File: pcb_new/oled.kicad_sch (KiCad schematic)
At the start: 33 parts, among them J10 3-2328724-1, U8 TPS6734ID

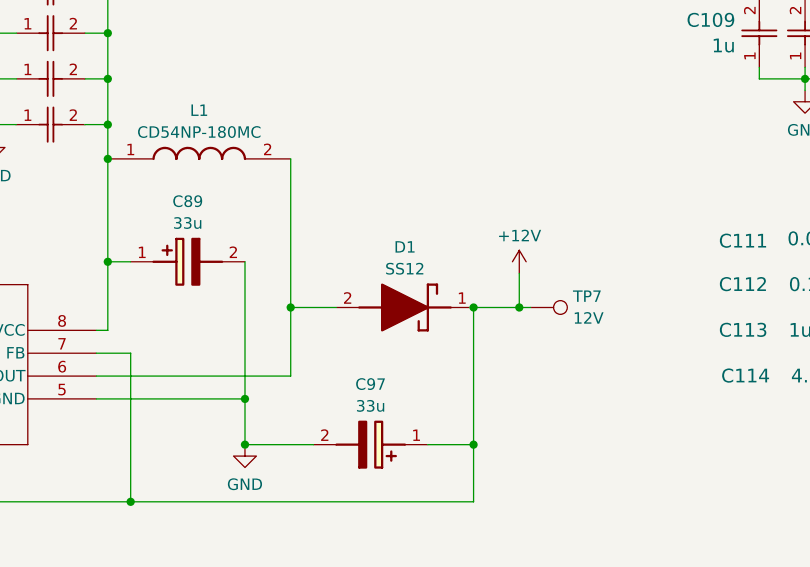
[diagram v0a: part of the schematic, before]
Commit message: initial test of new board
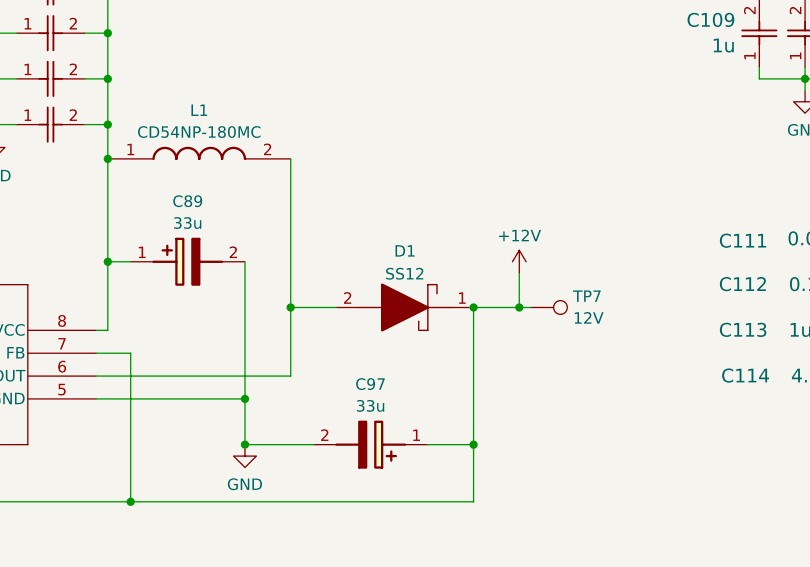
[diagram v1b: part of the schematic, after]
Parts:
- removed D1: SS12, OroLink:DIOM5027X244N, symbol OroLink:SS12
- added D1: SS12, OroLink:DIOM5027X244N, symbol SamacSys_Parts:SS12
- C105, C114, C115, C148: Mouser Part Number 81-GRM15C61E475ME15J -> (none)
- C89, C97: Mouser Part Number (none) -> 74-293D336X0020D2TE3; Mouser Price/Stock (none) -> https://www.mouser.de/ProductDetail/Vishay-Sprague/293D336X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
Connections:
- net +12V: now also D1.1
- net at L1.2, U8.6 (OUT): now also D1.2
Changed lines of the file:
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@@
 	)
 	(junction
-		(at 156.21 104.14)
-		(diameter 0)
-		(color 0 0 0 0)
-	)
-	(junction
 		(at 102.87 78.74)
 		(diameter 0)
@@
 	)
 	(junction
+		(at 156.21 104.14)
+		(diameter 0)
+		(color 0 0 0 0)
+	)
+	(junction
 		(at 243.84 120.65)
 		(diameter 0)
@@
 			)
 		)
-		(property "Mouser Part Number" "81-GRM15C61E475ME15J"
+		(property "Mouser Part Number" ""
 			(at 238.76 746.99 0)
 			(effects
@@
 	)
 	(symbol
-		(lib_id "OroLink:SS12")
-		(at 158.75 104.14 180)
-		(unit 1)
-		(exclude_from_sim no)
-		(in_bom yes)
-		(on_board yes)
-		(dnp no)
-		(fields_autoplaced yes)
-		(property "Reference" "D1"
-			(at 148.59 97.4555 0)
-			(effects
-				(font
-					(size 1.27 1.27)
-				)
-			)
-		)
-		(property "Value" "SS12"
-			(at 148.59 99.8798 0)
-			(effects
-				(font
-					(size 1.27 1.27)
-				)
-			)
-		)
-		(property "Footprint" "OroLink:DIOM5027X244N"
-			(at 146.05 10.49 0)
-			(effects
-				(font
-					(size 1.27 1.27)
-				)
-				(justify left top)
-				(hide yes)
-			)
-		)
-		(property "Datasheet" "https://www.panjit.com.tw/en/Product/downloadPDF/SS12"
-			(at 146.05 -89.51 0)
-			(effects
-				(font
-					(size 1.27 1.27)
-				)
-				(justify left top)
-				(hide yes)
-			)
-		)
-		(property "Description" "Power Schottky (IF1A) - SS12 , Standard, 20V, 1A, SMA"
-			(at 158.75 104.14 0)
-			(effects
-				(font
-					(size 1.27 1.27)
-				)
-				(hide yes)
-			)
-		)
-		(property "Height" "2.44"
-			(at 146.05 -289.51 0)
-			(effects
-				(font
-					(size 1.27 1.27)
-				)
-				(justify left top)
-				(hide yes)
-			)
-		)
-		(property "Manufacturer_Name" "PANJIT"
-			(at 146.05 -389.51 0)
-			(effects
-				(font
-					(size 1.27 1.27)
-				)
-				(justify left top)
-				(hide yes)
-			)
-		)
-		(property "Manufacturer_Part_Number" "SS12"
-			(at 146.05 -489.51 0)
-			(effects
-				(font
-					(size 1.27 1.27)
-				)
-				(justify left top)
-				(hide yes)
-			)
-		)
-		(property "Mouser Part Number" ""
-			(at 146.05 -589.51 0)
-			(effects
-				(font
-					(size 1.27 1.27)
-				)
-				(justify left top)
-				(hide yes)
-			)
-		)
-		(property "Mouser Price/Stock" ""
-			(at 146.05 -689.51 0)
-			(effects
-				(font
-					(size 1.27 1.27)
-				)
-				(justify left top)
-				(hide yes)
-			)
-		)
-		(property "Arrow Part Number" ""
-			(at 146.05 -789.51 0)
-			(effects
-				(font
-					(size 1.27 1.27)
-				)
-				(justify left top)
-				(hide yes)
-			)
-		)
-		(property "Arrow Price/Stock" ""
-			(at 146.05 -889.51 0)
-			(effects
-				(font
-					(size 1.27 1.27)
-				)
-				(justify left top)
-				(hide yes)
-			)
-		)
-		(pin "2"
-		)
-		(pin "1"
-		)
-		(instances
-			(project ""
-				(path "/b8dafc19-6de0-4c8f-9903-23372e5103df/222205f2-0600-4315-a593-542b8c55a37e"
-					(reference "D1")
-					(unit 1)
-				)
-			)
-		)
-	)
-	(symbol
 		(lib_id "OroLink:C1608X5R1H102K080AA")
 		(at 80.01 125.73 0)
@@
 	)
 	(symbol
+		(lib_name "293D336X0020D2TE3_1")
 		(lib_id "OroLink:293D336X0020D2TE3")
 		(at 118.11 99.06 0)
@@
 			)
 		)
-		(property "Mouser Part Number" ""
+		(property "Mouser Part Number" "74-293D336X0020D2TE3"
 			(at 127 795.25 0)
 			(effects
@@
 			)
 		)
-		(property "Mouser Price/Stock" ""
+		(property "Mouser Price/Stock" "https://www.mouser.de/ProductDetail/Vishay-Sprague/293D336X0020D2TE3?qs=CSo7yzBSerDt4rQKYL2h%252Bw%3D%3D"
 			(at 127 895.25 0)
 			(effects
@@
 			)
 		)
-		(property "Mouser Part Number" "81-GRM15C61E475ME15J"
+		(property "Mouser Part Number" ""
 			(at 210.82 807.95 0)
 			(effects
@@
 			)
 		)
-		(property "Mouser Part Number" "81-GRM15C61E475ME15J"
+		(property "Mouser Part Number" ""
 			(at 889.23 68.58 0)
 			(effects
@@
 	)
 	(symbol
+		(lib_id "SamacSys_Parts:SS12")
+		(at 158.75 104.14 180)
+		(unit 1)
+		(exclude_from_sim no)
+		(in_bom yes)
+		(on_board yes)
+		(dnp no)
+		(fields_autoplaced yes)
+		(property "Reference" "D1"
+			(at 148.59 97.9002 0)
+			(effects
+				(font
+					(size 1.27 1.27)
+				)
+			)
+		)
+		(property "Value" "SS12"
+			(at 148.59 100.4371 0)
+			(effects
+				(font
+					(size 1.27 1.27)
+				)
+			)
+		)
+		(property "Footprint" "OroLink:DIOM5027X244N"
+			(at 146.05 107.95 0)
+			(effects
+				(font
+					(size 1.27 1.27)
+				)
+				(justify left)
+				(hide yes)
+			)
+		)
+		(property "Datasheet" "https://datasheet.datasheetarchive.com/originals/distributors/Datasheets-24/DSA-463612.pdf"
+			(at 146.05 105.41 0)
+			(effects
+				(font
+					(size 1.27 1.27)
+				)
+				(justify left)
+				(hide yes)
+			)
+		)
+		(property "Description" "ON Semi SS12 SMT Schottky Diode, 20V 1A, 2-Pin DO-214AC"
+			(at 146.05 102.87 0)
+			(effects
+				(font
+					(size 1.27 1.27)
+				)
+				(justify left)
+				(hide yes)
+			)
+		)
+		(property "Height" "2.5"
+			(at 146.05 100.33 0)
+			(effects
+				(font
+					(size 1.27 1.27)
+				)
+				(justify left)
+				(hide yes)
+			)
+		)
+		(property "Manufacturer_Name" "onsemi"
+			(at 146.05 97.79 0)
+			(effects
+				(font
+					(size 1.27 1.27)
+				)
+				(justify left)
+				(hide yes)
+			)
+		)
+		(property "Manufacturer_Part_Number" "821-SS12"
+			(at 146.05 95.25 0)
+			(effects
+				(font
+					(size 1.27 1.27)
+				)
+				(justify left)
+				(hide yes)
+			)
+		)
+		(property "Mouser Part Number" "821-SS12"
+			(at 146.05 92.71 0)
+			(effects
+				(font
+					(size 1.27 1.27)
+				)
+				(justify left)
+				(hide yes)
+			)
+		)
+		(property "Mouser Price/Stock" "https://www.mouser.co.uk/ProductDetail/ON-Semiconductor-Fairchild/SS12?qs=mVVXn4M53U9WoaEpU1CO0A%3D%3D"
+			(at 146.05 90.17 0)
+			(effects
+				(font
+					(size 1.27 1.27)
+				)
+				(justify left)
+				(hide yes)
+			)
+		)
+		(property "Arrow Part Number" "SS12"
+			(at 146.05 87.63 0)
+			(effects
+				(font
+					(size 1.27 1.27)
+				)
+				(justify left)
+				(hide yes)
+			)
+		)
+		(property "Arrow Price/Stock" "https://www.arrow.com/en/products/ss12/on-semiconductor?region=nac"
+			(at 146.05 85.09 0)
+			(effects
+				(font
+					(size 1.27 1.27)
+				)
+				(justify left)
+				(hide yes)
+			)
+		)
+		(property "Mouser Testing Part Number" ""
+			(at 146.05 82.55 0)
+			(effects
+				(font
+					(size 1.27 1.27)
+				)
+				(justify left)
+				(hide yes)
+			)
+		)
+		(property "Mouser Testing Price/Stock" ""
+			(at 146.05 80.01 0)
+			(effects
+				(font
+					(size 1.27 1.27)
+				)
+				(justify left)
+				(hide yes)
+			)
+		)
+		(pin "1"
+		)
+		(pin "2"
+		)
+		(instances
+			(project "link"
+				(path "/b8dafc19-6de0-4c8f-9903-23372e5103df/222205f2-0600-4315-a593-542b8c55a37e"
+					(reference "D1")
+					(unit 1)
+				)
+			)
+		)
+	)
+	(symbol
 		(lib_id "OroLink:293D336X0020D2TE3")
 		(at 151.13 119.38 180)
@@
 			)
 		)
-		(property "Mouser Part Number" ""
+		(property "Mouser Part Number" "74-293D336X0020D2TE3"
 			(at 142.24 -576.81 0)
 			(effects
@@
 			)
 		)
-		(property "Mouser Price/Stock" ""
+		(property "Mouser Price/Stock" "https://www.mouser.de/ProductDetail/Vishay-Sprague/293D336X0020D2TE3?qs=CSo7yzBSerDt4rQKYL2h%252Bw%3D%3D"
 			(at 142.24 -676.81 0)
 			(effects
@@
 			)
 		)
-		(property "Mouser Part Number" "81-GRM15C61E475ME15J"
+		(property "Mouser Part Number" ""
 			(at 114.3 780.01 0)
 			(effects
